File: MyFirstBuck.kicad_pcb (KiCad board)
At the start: 2 copper layers, 130.8 x 132.1 mm, 50 parts, among them J1 Conn_01x01_Pin, J2 Conn_01x01_Pin, J3 Conn_01x01_Pin, J4 Conn_01x01_Pin, J5 Conn_01x01_Pin, Q1 IRF540NPBF, U1 LM358AP, U2 LAUNCHXL-F28379D, U3 UCC5304DWVR, U4 TMV 0512SHI

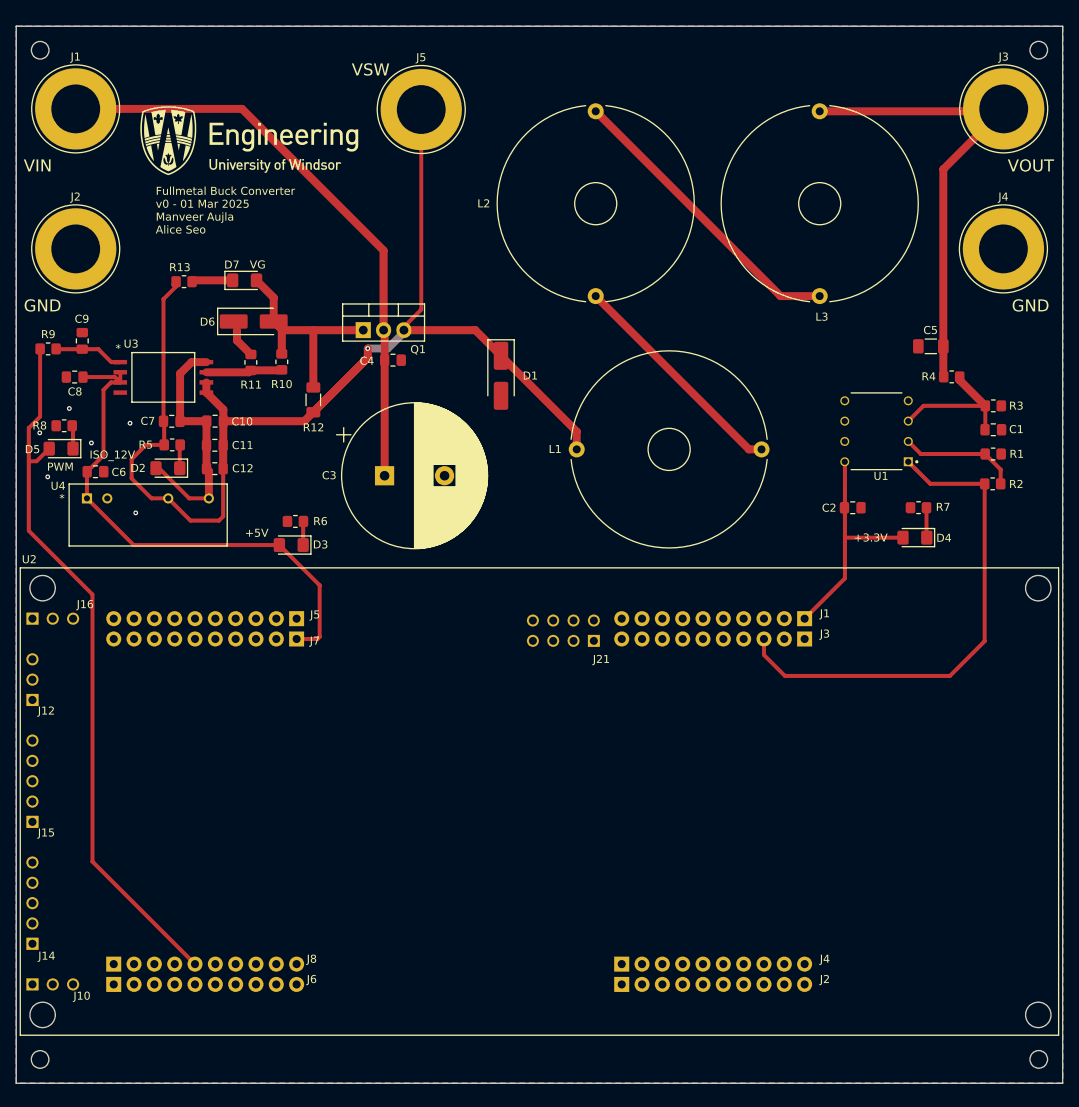
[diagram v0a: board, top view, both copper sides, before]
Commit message: Add files via upload
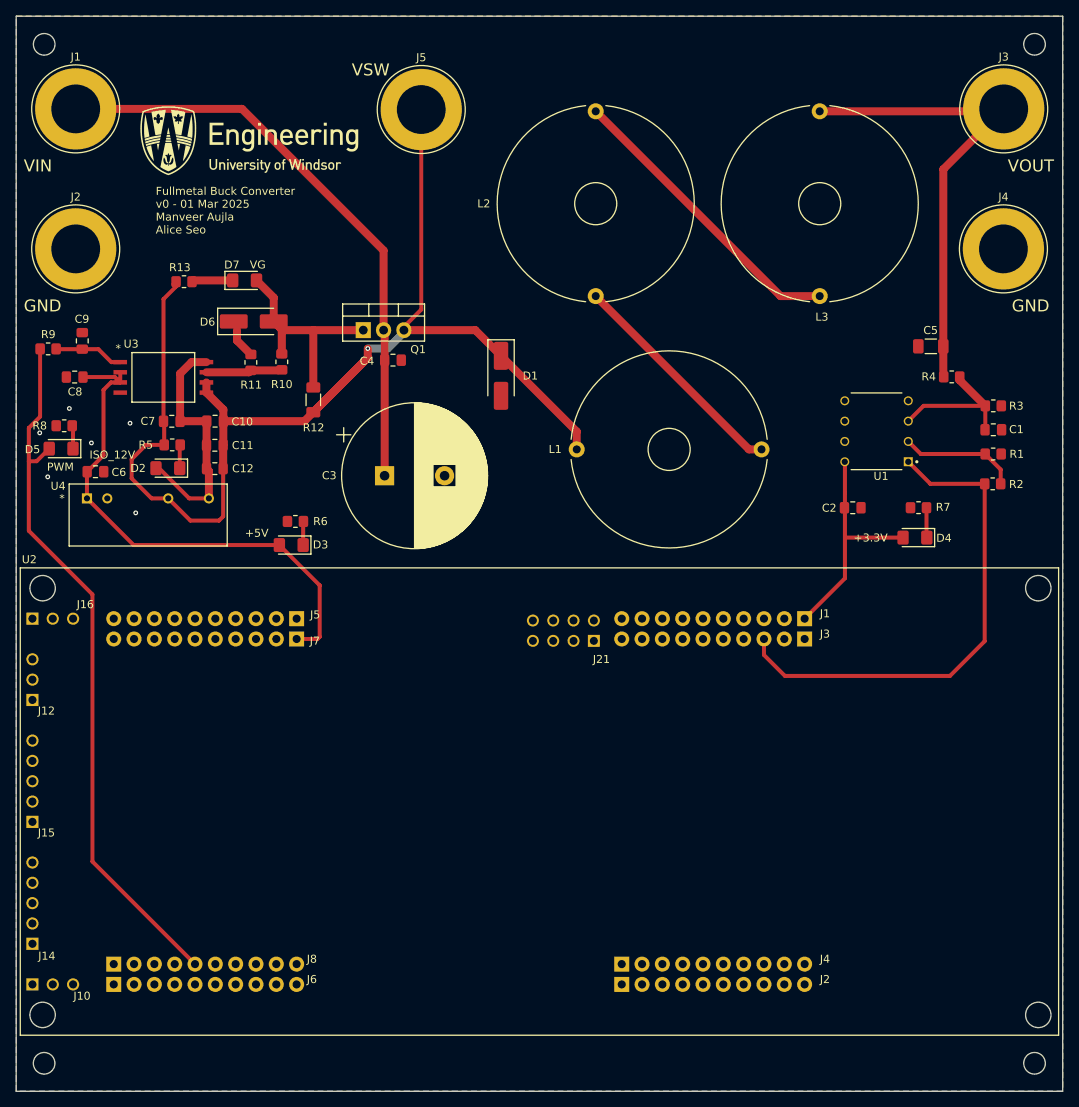
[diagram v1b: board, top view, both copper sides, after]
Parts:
- removed the REF** at (163.4, 180.3)
- removed the REF** at (163.4, 54.2)
- removed the REF** at (38.6, 54.2)
- removed the REF** at (38.5, 180.3)
- added REF**: MountingHole_2.7mm_M2.5, MountingHole:MountingHole_2.7mm_M2.5, F.Cu at (162.8, 180.8)
- added REF**: MountingHole_2.7mm_M2.5, MountingHole:MountingHole_2.7mm_M2.5, F.Cu at (39.0, 180.8)
- added REF**: MountingHole_2.7mm_M2.5, MountingHole:MountingHole_2.7mm_M2.5, F.Cu at (162.8, 53.4)
- added REF**: MountingHole_2.7mm_M2.5, MountingHole:MountingHole_2.7mm_M2.5, F.Cu at (39.1, 53.4)
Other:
- board size 130.8 x 132.1 mm -> 130.8 x 134.4 mm
